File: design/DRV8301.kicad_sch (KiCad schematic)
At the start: 38 parts, among them U2 MC74VHC1GT66, U3 MC74VHC1GT66, U4 MC74VHC1GT66

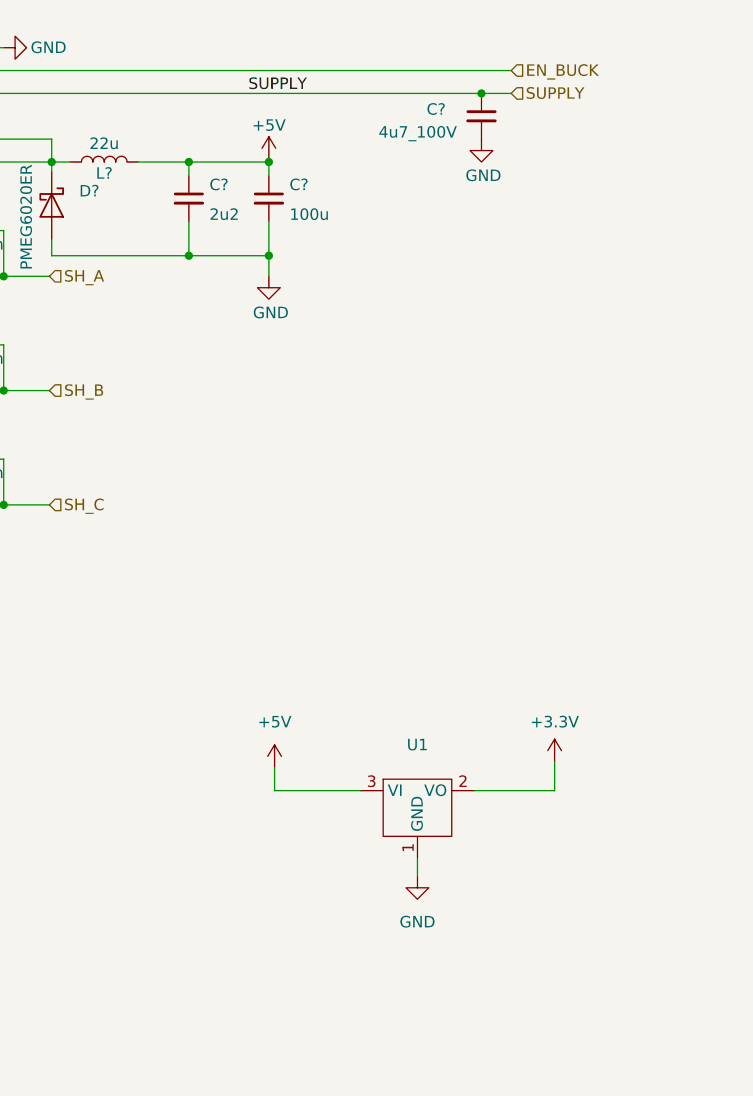
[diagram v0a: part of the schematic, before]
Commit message: more BLDC updates
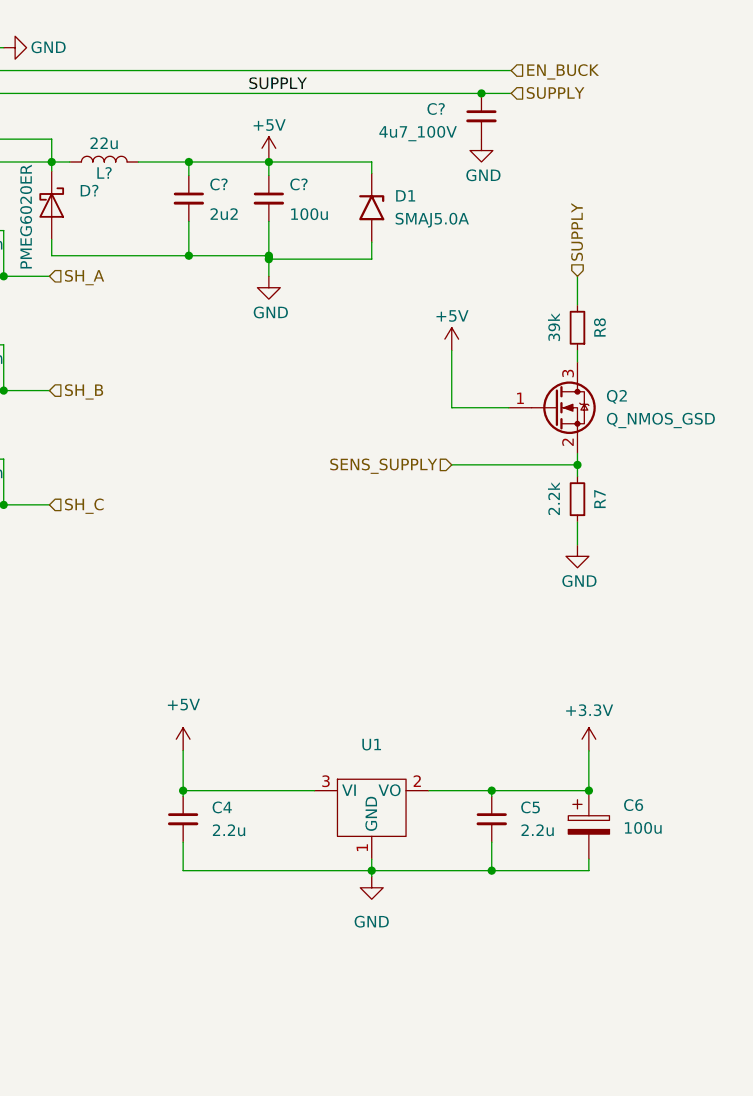
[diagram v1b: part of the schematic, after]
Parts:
- added C4, C5: 2.2u, symbol Device:C_Small
- added C6: 100u, symbol Device:C_Polarized
- added D1: SMAJ5.0A, Diode_SMD:D_SMA, symbol Diode:SMAJ5.0A
- added Q2: Q_NMOS_GSD, symbol Device:Q_NMOS_GSD
- added R7: 2.2k, Resistor_SMD:R_0603_1608Metric_Pad0.98x0.95mm_HandSolder, symbol Device:R_Small
- added R8: 39k, Resistor_SMD:R_0603_1608Metric_Pad0.98x0.95mm_HandSolder, symbol Device:R_Small
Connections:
- net +3.3V: now also C5.1, C6.1
- net +5V: now also C4.1, D1.1 (A1), Q2.1 (G)
- net GND: now also C4.2, C5.2, C6.2, D1.2 (A2), R7.1
- net SUPPLY: now also R8.2
- new net: Q2.3 (D), R8.1
- new net SENS_SUPPLY: Q2.2 (S), R7.2
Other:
- moved on the sheet: U1
